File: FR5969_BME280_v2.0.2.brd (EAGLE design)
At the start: 9.2 x 10.7 mm, 13 parts, among them U1 MSP430FR5969, U2 BME280

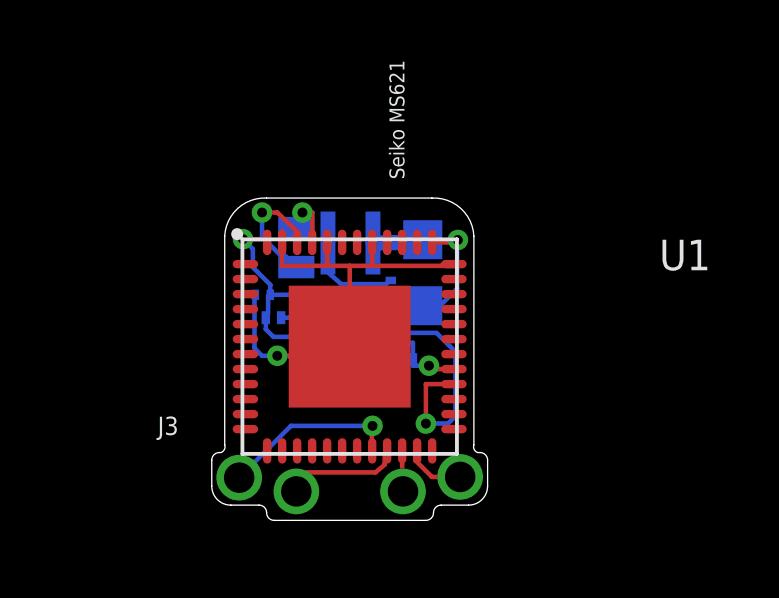
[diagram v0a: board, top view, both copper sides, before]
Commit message: Update FR5969_BME280_v2.0.2.brd
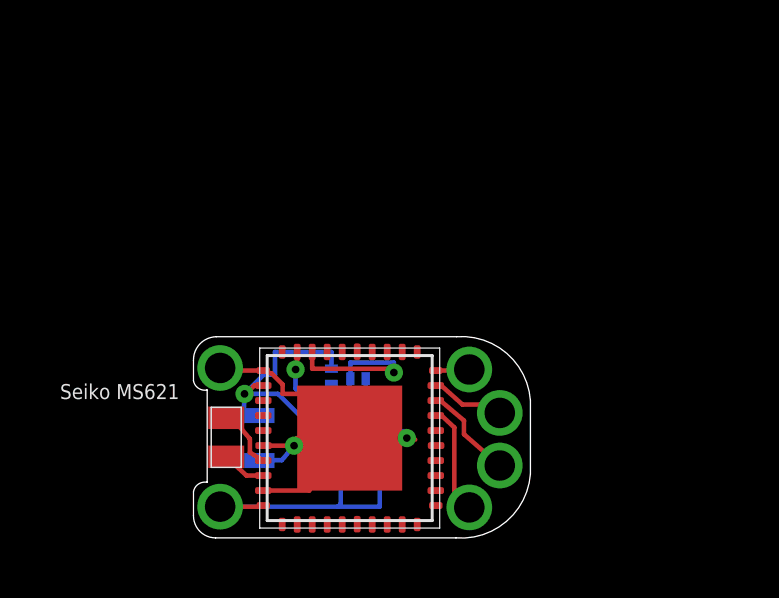
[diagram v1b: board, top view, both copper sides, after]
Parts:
- removed C1, C2: 100 pF, resistor:C0201
- removed SEIKO-MS621: 5.5 mAh, battery:SEIKO_MICRO
- removed U2: BME280, BME280ComponentLibrary:BME280_LGA
- added J5: TEST, SparkFun-Connectors:1X01
- added J6: RESET, SparkFun-Connectors:1X01
- added U$3: SEIKO-MS621, battery:SEIKO_MICRO
- J1: value (none) -> VSS
- J2: value (none) -> VCC
- J3: value (none) -> TXD
- J4: value (none) -> RXD
- U$1: value CPX3225 -> MSP430FR5949_RHA; device seiko:CPX3225_CHIP-CAP -> chips:RHA-40-VQFN
- U1: value MSP430FR5969 -> BME280; device chips:S-PVQFN-N48 -> BME280ComponentLibrary:BME280_LGA
- moved J2 8.06 mm to (0.76, 1.02), flipped to the top
- moved J3 7.73 mm to (9.07, 0.99), flipped to the top
- moved J1 7.35 mm to (0.76, 5.64), flipped to the top
- moved J4 6.84 mm to (10.1, 2.39), flipped to the top
- moved U$2 6.74 mm to (0.97, 3.33), flipped to the top, turned to 90 degrees
- moved U$1 6.03 mm to (5.08, 3.30), flipped to the top, turned to 0 degrees
- moved U1 3.02 mm to (5.11, 3.33), flipped to the bottom, turned to 90 degrees
- moved R2 2.75 mm to (4.47, 5.36), turned to 270 degrees
- moved R1 1.70 mm to (5.36, 5.28)
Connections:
- removed net BATT+: SEIKO-MS621.1-POS, U$1.2
- removed net GND: C1.2, C2.2, SEIKO-MS621.2-GND, U1.36, U1.41, U1.44, U1.47, U1.49, U2.P$1, U2.P$7
- removed net N$1: U$2.2-XTI, U1.46
- removed net N$2: U$2.1-XTO, U1.45
- removed net RX: J4.1, U1.21
- removed net TX: J3.1, U1.20
- new net RXD: J4.1, U$1.18
- new net TXD: J3.1, U$1.17
- new net VSS: J1.1, U$1.31, U$1.36, U$1.39, U$3.2-GND, U1.P$1, U1.P$7
- new net XTAL_IN: U$1.37, U$2.2-XTI
- new net XTAL_OUT: U$1.38, U$2.1-XTO
- net RESET: now also J6.1, U$1.20; no longer J2.1, U1.23
- net SCL: now also R2.2, U$1.29, U1.P$4; no longer R2.1, U1.28, U2.P$4
- net SDA: now also R1.2, U$1.28, U1.P$3; no longer R1.1, U1.29, U2.P$3
- net TEST: now also J5.1, U$1.19; no longer J1.1, U1.22
- net VCC: now also J2.1, R1.1, R2.1, U$1.32, U$1.40, U$3.1-POS, U1.P$2, U1.P$6, U1.P$8; no longer C1.1, C2.1, R1.2, R2.2, U$1.1, U1.37, U1.48, U2.P$2, U2.P$6, U2.P$8
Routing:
- net GND: track 27.4 -> 0.00 mm, vias 1 -> 0
- net VSS: track 0.00 -> 19.3 mm, vias 0 -> 2
- net SCL: track 12.6 -> 3.41 mm
- net TX: track 6.11 -> 0.00 mm, vias 1 -> 0
- net RX: track 4.17 -> 0.00 mm
- net N$1: track 4.15 -> 0.00 mm, vias 1 -> 0
- net TXD: track 0.00 -> 3.65 mm
- net RXD: track 0.00 -> 3.24 mm
- net SDA: track 3.62 -> 6.80 mm
- net XTAL_IN: track 0.00 -> 2.08 mm
- net N$2: track 1.89 -> 0.00 mm, vias 1 -> 0
- net VCC: track 20.8 -> 22.6 mm, vias 2 -> 1
- net BATT+: track 1.68 -> 0.00 mm
- net XTAL_OUT: track 0.00 -> 1.48 mm
- net TEST: track 1.36 -> 2.45 mm
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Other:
- board size 9.2 x 10.7 mm -> 11.2 x 6.7 mm
